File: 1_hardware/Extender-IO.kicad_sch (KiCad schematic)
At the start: 8 parts, among them U10 PCA9555PW,118, U11 PCA9555PW,118, U4 PCA9555PW,118, U5 PCA9555PW,118, U6 PCA9555PW,118, U7 PCA9555PW,118, U8 PCA9555PW,118, U9 PCA9555PW,118

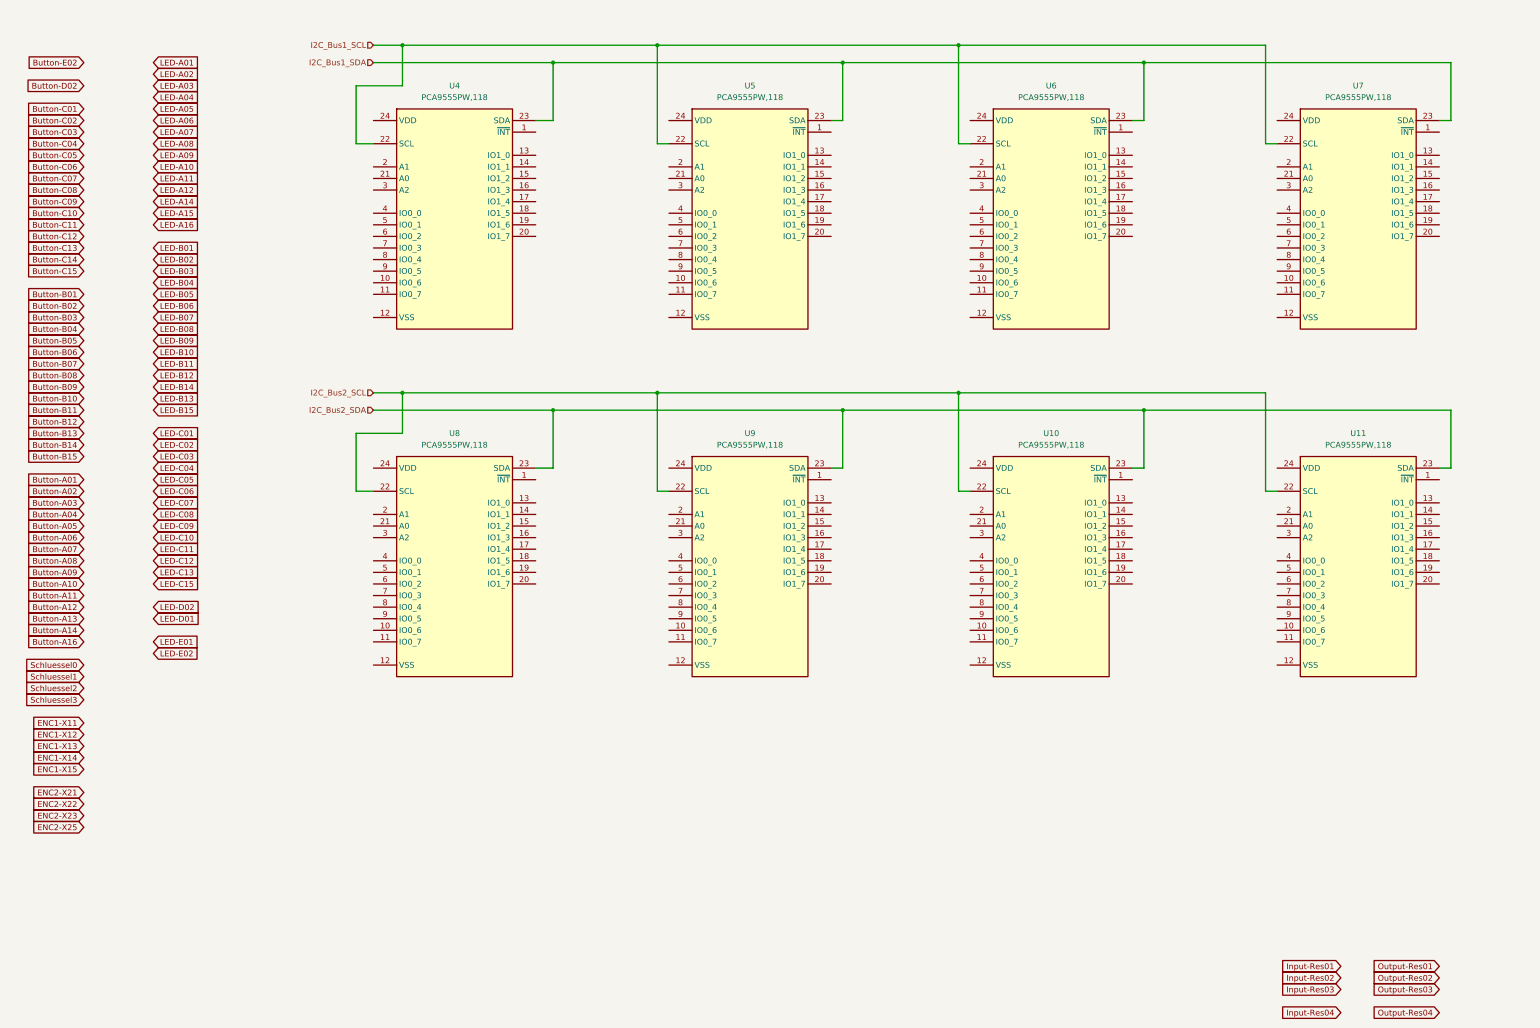
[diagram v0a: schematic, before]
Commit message: finished schematics and board
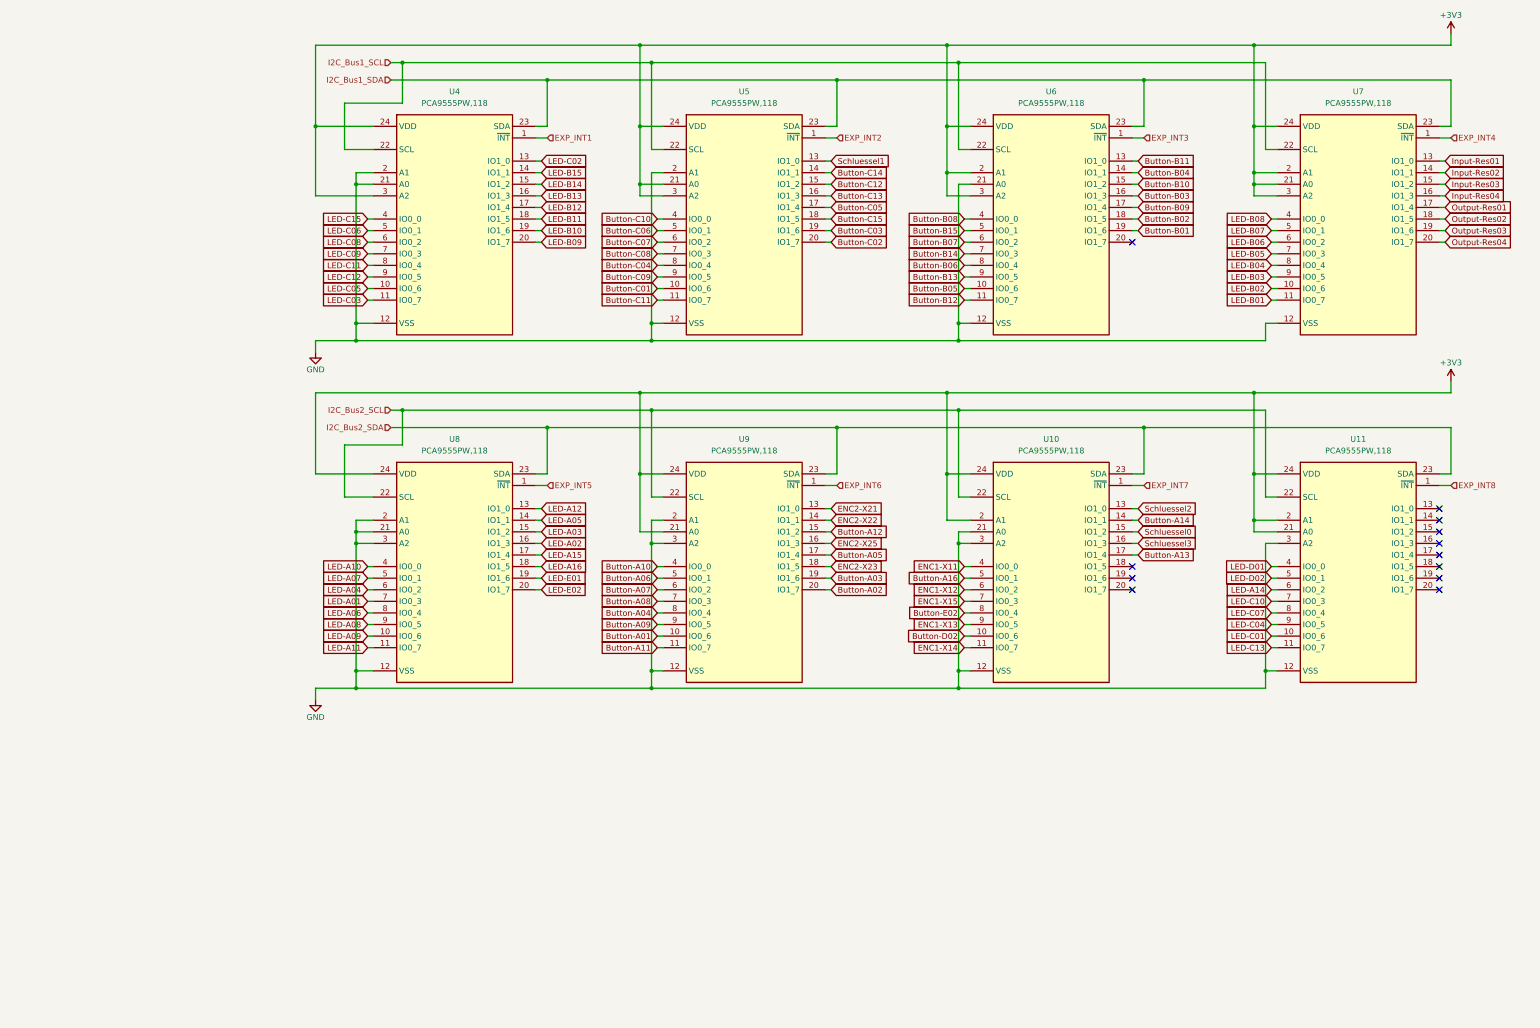
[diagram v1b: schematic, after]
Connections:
- net Button-A01: now also U9.10 (IO0_6)
- net Button-A02: now also U9.20 (IO1_7)
- net Button-A03: now also U9.19 (IO1_6)
- net Button-A04: now also U9.8 (IO0_4)
- net Button-A05: now also U9.17 (IO1_4)
- net Button-A06: now also U9.5 (IO0_1)
- net Button-A07: now also U9.6 (IO0_2)
- net Button-A08: now also U9.7 (IO0_3)
- net Button-A09: now also U9.9 (IO0_5)
- net Button-A10: now also U9.4 (IO0_0)
- net Button-A11: now also U9.11 (IO0_7)
- net Button-A12: now also U9.15 (IO1_2)
- net Button-A13: now also U10.17 (IO1_4)
- net Button-A14: now also U10.14 (IO1_1)
- net Button-A16: now also U10.5 (IO0_1)
- net Button-B01: now also U6.19 (IO1_6)
- net Button-B02: now also U6.18 (IO1_5)
- net Button-B03: now also U6.16 (IO1_3)
- net Button-B04: now also U6.14 (IO1_1)
- net Button-B05: now also U6.10 (IO0_6)
- net Button-B06: now also U6.8 (IO0_4)
- net Button-B07: now also U6.6 (IO0_2)
- net Button-B08: now also U6.4 (IO0_0)
- net Button-B09: now also U6.17 (IO1_4)
- net Button-B10: now also U6.15 (IO1_2)
- net Button-B11: now also U6.13 (IO1_0)
- net Button-B12: now also U6.11 (IO0_7)
- net Button-B13: now also U6.9 (IO0_5)
- net Button-B14: now also U6.7 (IO0_3)
- net Button-B15: now also U6.5 (IO0_1)
- net Button-C01: now also U5.10 (IO0_6)
- net Button-C02: now also U5.20 (IO1_7)
- net Button-C03: now also U5.19 (IO1_6)
- net Button-C04: now also U5.8 (IO0_4)
- net Button-C05: now also U5.17 (IO1_4)
- net Button-C06: now also U5.5 (IO0_1)
- net Button-C07: now also U5.6 (IO0_2)
- net Button-C08: now also U5.7 (IO0_3)
- net Button-C09: now also U5.9 (IO0_5)
- net Button-C10: now also U5.4 (IO0_0)
- net Button-C11: now also U5.11 (IO0_7)
- net Button-C12: now also U5.15 (IO1_2)
- net Button-C13: now also U5.16 (IO1_3)
- net Button-C14: now also U5.14 (IO1_1)
- net Button-C15: now also U5.18 (IO1_5)
- net Button-D02: now also U10.10 (IO0_6)
- net Button-E02: now also U10.8 (IO0_4)
- net ENC1-X11: now also U10.4 (IO0_0)
- net ENC1-X12: now also U10.6 (IO0_2)
- net ENC1-X13: now also U10.9 (IO0_5)
- net ENC1-X14: now also U10.11 (IO0_7)
- net ENC1-X15: now also U10.7 (IO0_3)
- net ENC2-X21: now also U9.13 (IO1_0)
- net ENC2-X22: now also U9.14 (IO1_1)
- net ENC2-X23: now also U9.18 (IO1_5)
- net ENC2-X25: now also U9.16 (IO1_3)
- net Input-Res01: now also U7.13 (IO1_0)
- net Input-Res02: now also U7.14 (IO1_1)
- net Input-Res03: now also U7.15 (IO1_2)
- net Input-Res04: now also U7.16 (IO1_3)
- net LED-A01: now also U8.7 (IO0_3)
- net LED-A02: now also U8.16 (IO1_3)
- net LED-A03: now also U8.15 (IO1_2)
- net LED-A04: now also U8.6 (IO0_2)
- net LED-A05: now also U8.14 (IO1_1)
- net LED-A06: now also U8.8 (IO0_4)
- net LED-A07: now also U8.5 (IO0_1)
- net LED-A08: now also U8.9 (IO0_5)
- net LED-A09: now also U8.10 (IO0_6)
- net LED-A10: now also U8.4 (IO0_0)
- net LED-A11: now also U8.11 (IO0_7)
- net LED-A12: now also U8.13 (IO1_0)
- net LED-A14: now also U11.6 (IO0_2)
- net LED-A15: now also U8.17 (IO1_4)
- net LED-A16: now also U8.18 (IO1_5)
- net LED-B01: now also U7.11 (IO0_7)
- net LED-B02: now also U7.10 (IO0_6)
- net LED-B03: now also U7.9 (IO0_5)
- net LED-B04: now also U7.8 (IO0_4)
- net LED-B05: now also U7.7 (IO0_3)
- net LED-B06: now also U7.6 (IO0_2)
- net LED-B07: now also U7.5 (IO0_1)
- net LED-B08: now also U7.4 (IO0_0)
- net LED-B09: now also U4.20 (IO1_7)
- net LED-B10: now also U4.19 (IO1_6)
- net LED-B11: now also U4.18 (IO1_5)
- net LED-B12: now also U4.17 (IO1_4)
- net LED-B13: now also U4.16 (IO1_3)
- net LED-B14: now also U4.15 (IO1_2)
- net LED-B15: now also U4.14 (IO1_1)
- net LED-C01: now also U11.10 (IO0_6)
- net LED-C02: now also U4.13 (IO1_0)
- net LED-C03: now also U4.11 (IO0_7)
- net LED-C04: now also U11.9 (IO0_5)
- net LED-C05: now also U4.10 (IO0_6)
- net LED-C06: now also U4.5 (IO0_1)
- net LED-C07: now also U11.8 (IO0_4)
- net LED-C08: now also U4.6 (IO0_2)
- net LED-C09: now also U4.7 (IO0_3)
- net LED-C10: now also U11.7 (IO0_3)
- net LED-C11: now also U4.8 (IO0_4)
- net LED-C12: now also U4.9 (IO0_5)
- net LED-C13: now also U11.11 (IO0_7)
- net LED-C15: now also U4.4 (IO0_0)
- net LED-D01: now also U11.4 (IO0_0)
- net LED-D02: now also U11.5 (IO0_1)
- net LED-E01: now also U8.19 (IO1_6)
- net LED-E02: now also U8.20 (IO1_7)
- net Output-Res01: now also U7.17 (IO1_4)
- net Output-Res02: now also U7.18 (IO1_5)
- net Output-Res03: now also U7.19 (IO1_6)
- net Output-Res04: now also U7.20 (IO1_7)
- net Schluessel0: now also U10.15 (IO1_2)
- net Schluessel1: now also U5.13 (IO1_0)
- net Schluessel2: now also U10.13 (IO1_0)
- net Schluessel3: now also U10.16 (IO1_3)
- net EXP_INT1: now reaches U4.1 (~{INT})
- net GND: now reaches U4.12 (VSS)
- net GND: now also U10.12 (VSS), U10.21 (A0), U10.3 (A2), U11.12 (VSS), U11.3 (A2), U4.2 (A1), U4.21 (A0), U5.12 (VSS), U5.2 (A1), U6.12 (VSS), U6.21 (A0), U7.12 (VSS), U8.12 (VSS), U8.2 (A1), U8.21 (A0), U8.3 (A2), U9.12 (VSS), U9.2 (A1), U9.3 (A2)
- net +3V3: now reaches U4.24 (VDD)
- net +3V3: now also U10.2 (A1), U10.24 (VDD), U11.2 (A1), U11.21 (A0), U11.24 (VDD), U4.3 (A2), U5.21 (A0), U5.24 (VDD), U5.3 (A2), U6.2 (A1), U6.24 (VDD), U6.3 (A2), U7.2 (A1), U7.21 (A0), U7.24 (VDD), U7.3 (A2), U8.24 (VDD), U9.21 (A0), U9.24 (VDD)
- net EXP_INT2: now reaches U5.1 (~{INT})
- net EXP_INT4: now reaches U7.1 (~{INT})
- net EXP_INT5: now reaches U8.1 (~{INT})
- net EXP_INT7: now reaches U10.1 (~{INT})
- net EXP_INT8: now reaches U11.1 (~{INT})
- net EXP_INT6: now reaches U9.1 (~{INT})
- net EXP_INT3: now reaches U6.1 (~{INT})
- no-connect marks 0 -> 12
